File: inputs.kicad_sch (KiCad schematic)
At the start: 36 parts, among them J10 Screw_Terminal_01x02, J9 Inputs, Q103 TLP521-4XSM, Q104 TLP521-4XSM

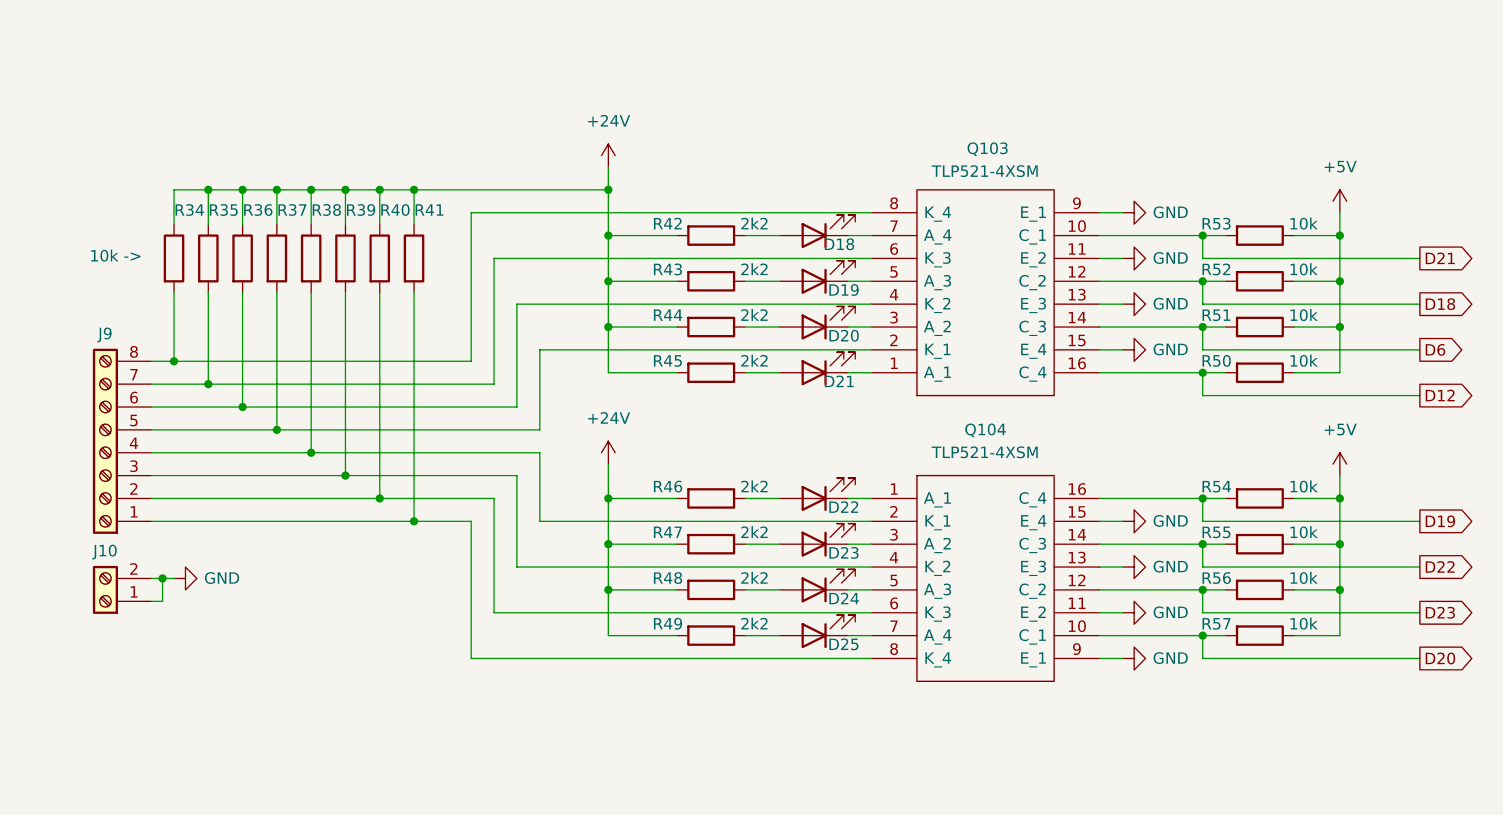
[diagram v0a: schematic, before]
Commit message: Made the PCK the size of the LP board
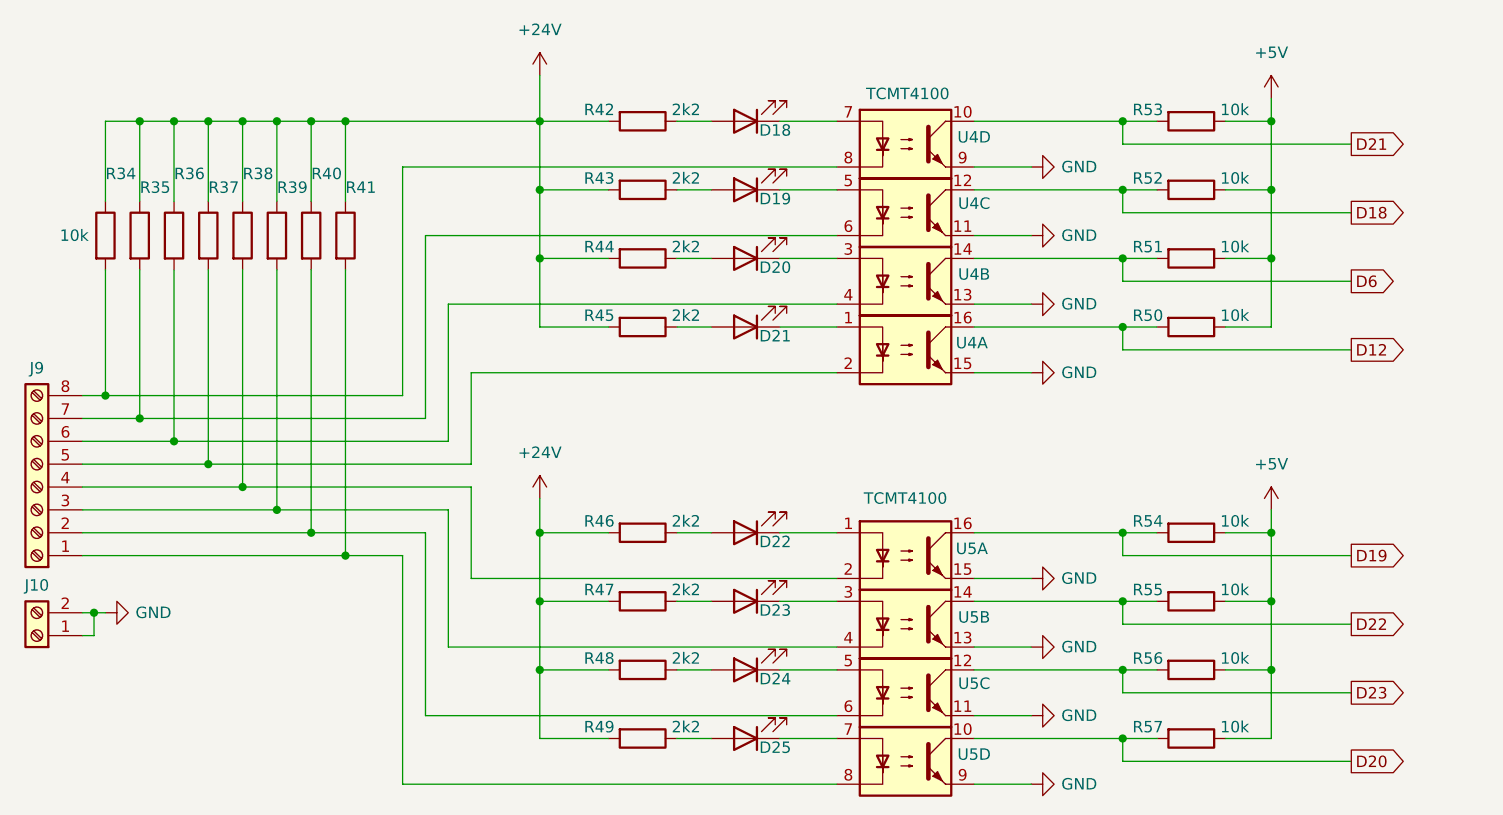
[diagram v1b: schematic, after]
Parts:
- removed Q103, Q104: TLP521-4XSM, SamacSys_Parts:TLP5214XSM, symbol SamacSys_Parts:TLP521-4XSM
- added U4, U5: TCMT4100, Package_SO:SOP-16_4.4x10.4mm_P1.27mm, symbol Isolator:TCMT4100
- R34: value 10k -> -> 10k
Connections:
- net D12: now also U4.16
- net D18: now also U4.12
- net D19: now also U5.16
- net D20: now also U5.10
- net D21: now also U4.10
- net D22: now also U5.14
- net D23: now also U5.12
- net D6: now also U4.14
- net GND: now also U4.11, U4.13, U4.15, U4.9, U5.11, U5.13, U5.15, U5.9
- net at D23.1 (K): now also U5.3
- net at D19.1 (K): now also U4.5
- net at D21.1 (K): now also U4.1
- net at J9.5 (Pin_5), R37.2: now also U4.2
- net at D20.1 (K): now also U4.3
- net at J9.6 (Pin_6), R36.2: now also U4.4
- net at J9.7 (Pin_7), R35.2: now also U4.6
- net at D18.1 (K): now also U4.7
- net at J9.8 (Pin_8), R34.2: now also U4.8
- net at D22.1 (K): now also U5.1
- net at D24.1 (K): now also U5.5
- net at J9.1 (Pin_1), R41.2: now also U5.8
- net at J9.2 (Pin_2), R40.2: now also U5.6
- net at J9.3 (Pin_3), R39.2: now also U5.4
- net at J9.4 (Pin_4), R38.2: now also U5.2
- net at D25.1 (K): now also U5.7
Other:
- moved on the sheet: D18, D19, D20, D21, D22, D23, D24, D25, J10, J9, R34, R35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
